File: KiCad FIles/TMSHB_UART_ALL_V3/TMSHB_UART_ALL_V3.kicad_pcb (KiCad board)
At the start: 2 copper layers, 309.9 x 264.2 mm, 128 parts, among them J1 Conn_01x08_Pin, J10 Conn_01x14_Pin, J11 Conn_01x14_Pin, J12 Conn_01x14_Pin, J13 Conn_01x15_Pin, J14 Conn_01x16_Pin, J15 Conn_01x16_Pin, J16 Conn_01x08_Pin, J17 Conn_01x05_Pin, J18 Conn_01x05_Pin, J19 Conn_01x05_Pin, J2 Conn_01x15_Pin, J20 Conn_01x15_Pin, J21 Conn_01x15_Pin, J22 Conn_01x16_Pin, J23 Conn_01x08_Pin, J24 Conn_01x05_Pin, J25 Conn_01x05_Pin, J26 Conn_01x05_Pin, J27 Conn_01x08_Pin, J28 Conn_01x05_Pin, J29 Conn_01x05_Pin, J3 Conn_01x16_Pin, J30 Conn_01x05_Pin, J31 Conn_01x14_Pin, J32 Conn_01x02_Pin, J33 Conn_01x14_Pin, J34 Conn_01x02_Pin, J35 Conn_01x14_Pin, J36 Conn_01x14_Pin, J37 Conn_01x14_Pin, J4 Conn_01x05_Pin, J5 Conn_01x05_Pin, J6 Conn_01x03_Pin, J7 Conn_01x05_Pin, J8 Conn_01x03_Pin, J9 Interconnect, Q1 NPN, Q13 NPN, Q14 PNP, Q2 PNP, Q3 NPN, Q4 NPN, Q5 NPN, Q6 NPN, U1 TR1602, U10 NE555P, U11 74LS138, U12 74LS148, U13 74LS138, U14 74LS00, U15 NE555P, U2 74LS04, U3 74LS00, U4 74LS32, U5 NE555P, U6 74LS00, U7 TR1602, U8 74LS00, U9 74LS32

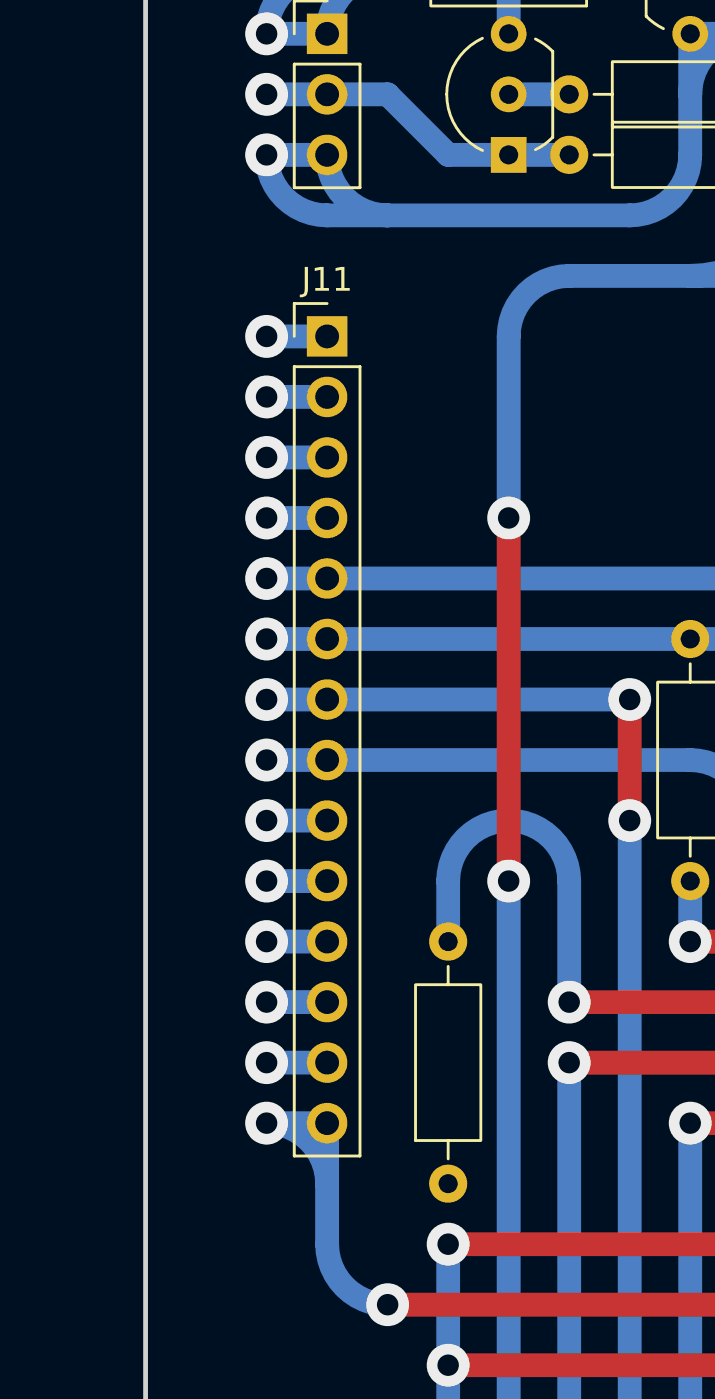
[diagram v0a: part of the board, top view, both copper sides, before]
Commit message: 2026/4/9
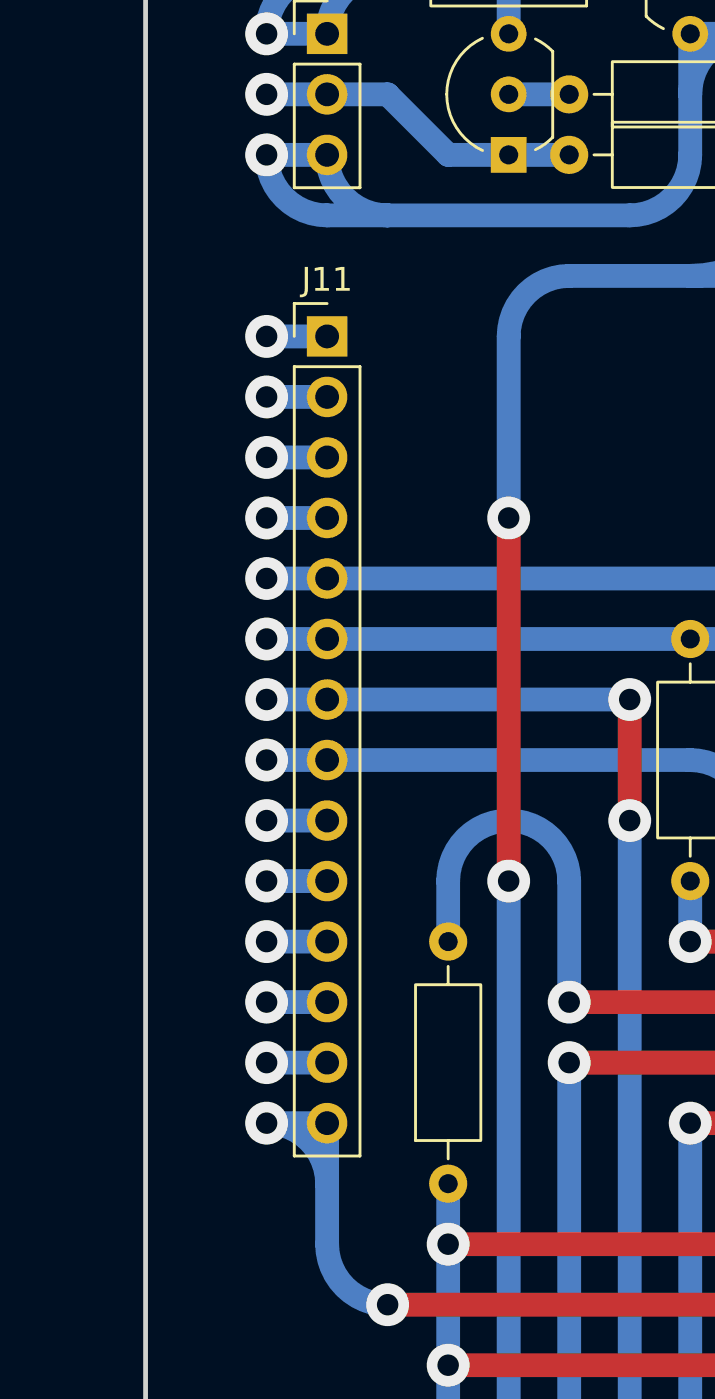
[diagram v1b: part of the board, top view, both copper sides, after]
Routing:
- net +5V: track 1548.6 -> 1551.2 mm
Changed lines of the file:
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@@
 	)
 	(segment
+		(start 256.54 256.54)
+		(end 256.54 254)
+		(width 1)
+		(layer "B.Cu")
+		(net 1)
+	)
+	(segment
 		(start 261.62 198.12)
 		(end 276.86 198.12)
@@
 	)
 	(segment
-		(start 254 213.36)
-		(end 251.46 213.36)
-		(width 1)
-		(layer "B.Cu")
-		(net 2)
-	)
-	(segment
 		(start 101.6 287.02)
 		(end 101.6 284.48)
@@
 	)
 	(segment
+		(start 251.46 213.36)
+		(end 254 213.36)
+		(width 1)
+		(layer "B.Cu")
+		(net 2)
+	)
+	(segment
 		(start 195.54 215.86)
 		(end 182.92 215.86)
@@
 	)
 	(arc
-		(start 251.46 213.36)
-		(mid 249.663949 212.616051)
-		(end 248.92 210.82)
-		(width 1)
-		(layer "B.Cu")
-		(net 2)
-	)
-	(arc
 		(start 322.58 266.7)
 		(mid 321.836051 268.496051)
@@
 		(width 1)
 		(layer "B.Cu")
+		(net 2)
+	)
+	(arc
+		(start 248.92 210.82)
+		(mid 249.663949 212.616051)
+		(end 251.46 213.36)
+		(width 1)
+		(layer "B.Cu")
